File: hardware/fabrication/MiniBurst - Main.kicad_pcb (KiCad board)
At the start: 2 copper layers, 65 x 128.5 mm, 79 parts, among them J1 TRIG_IN, J2 TRIG_OUT, J3 EXT_CLK, J4 DURATION_OUT, J5 END_OUT, J6 PULSES_OUT, J7 Conn_01x10_Pin, SW2 STEPS, SW3 SW_DPDT_x2, U1 LM358, U2 40106, U3 4017, U4 LM358, U5 LM358

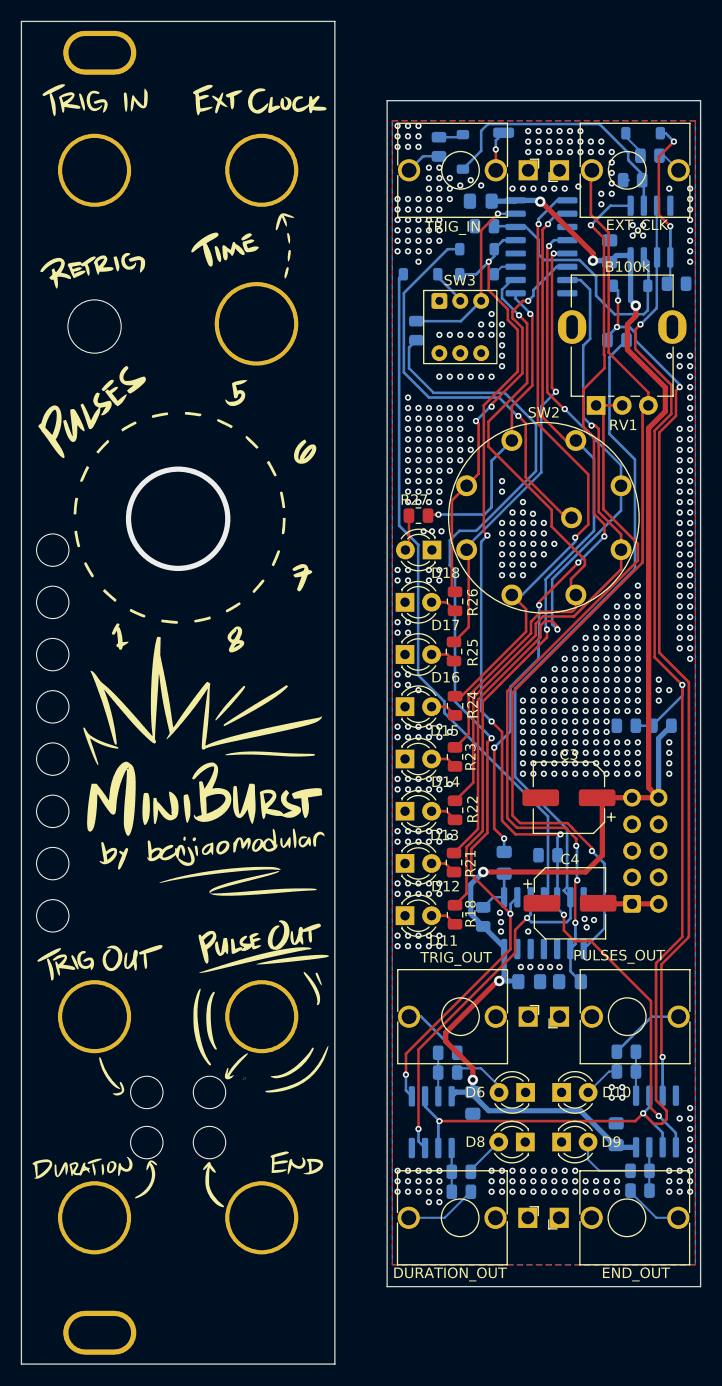
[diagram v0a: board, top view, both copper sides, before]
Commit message: v0.1 PCB
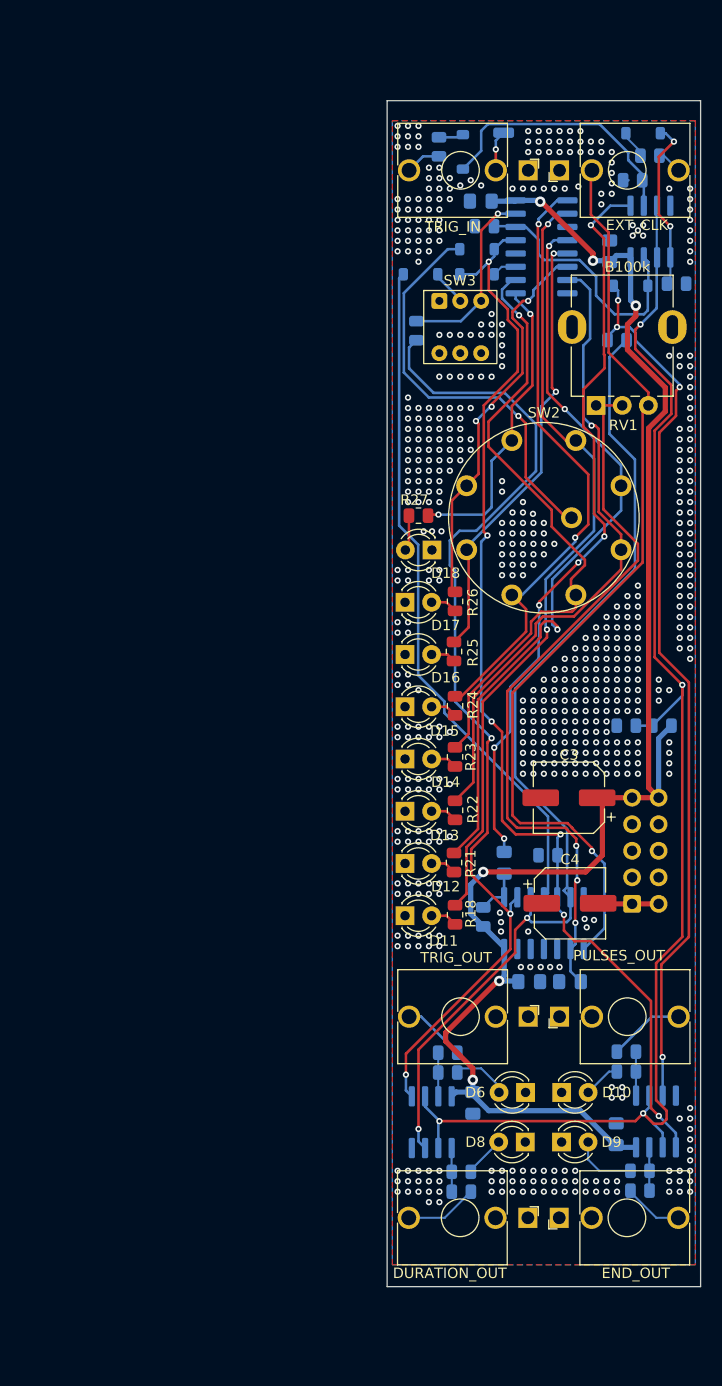
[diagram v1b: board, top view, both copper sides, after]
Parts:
- removed G***: LOGO, LOGO
- removed REF** (x6): PanelHole_AudioJack_3.5mm, benjiaomodular:PanelHole_AudioJack_3.5mm
- removed REF**: Panel_6HP, benjiaomodular:Panel_6HP
- removed REF**: PanelHole_Potentiometer_RV09, benjiaomodular:PanelHole_Potentiometer_RV09
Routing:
- net (no net): vias 14 -> 0
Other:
- board size 65 x 128.5 mm -> 30 x 113.5 mm
